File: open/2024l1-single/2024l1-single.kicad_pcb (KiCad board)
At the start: 2 copper layers, 176 x 169.5 mm, 100 parts, among them IC1 LM2587S-ADJ, J1 Conn_01x03, J2 Conn_01x03, J3 Conn_01x02, J4 Conn_01x02, J5 XT30, J6 Conn_01x04, Q1 STP75NF75, Q2 STP75NF75, U1 Seeed Studio XIAO SAMD21, U2 CD74HC4067SM

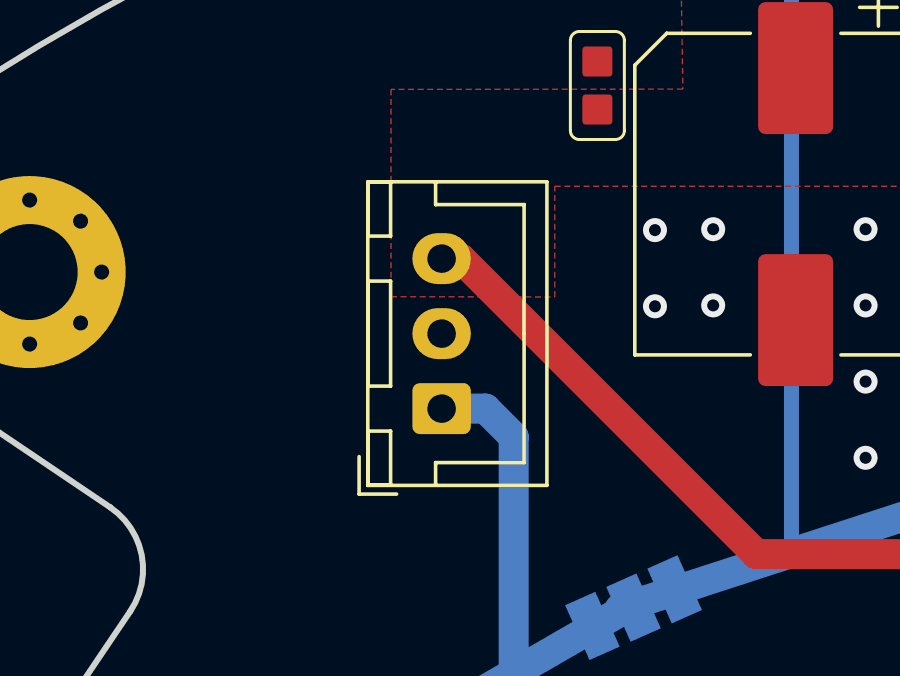
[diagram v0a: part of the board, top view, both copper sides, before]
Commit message: Connector movements
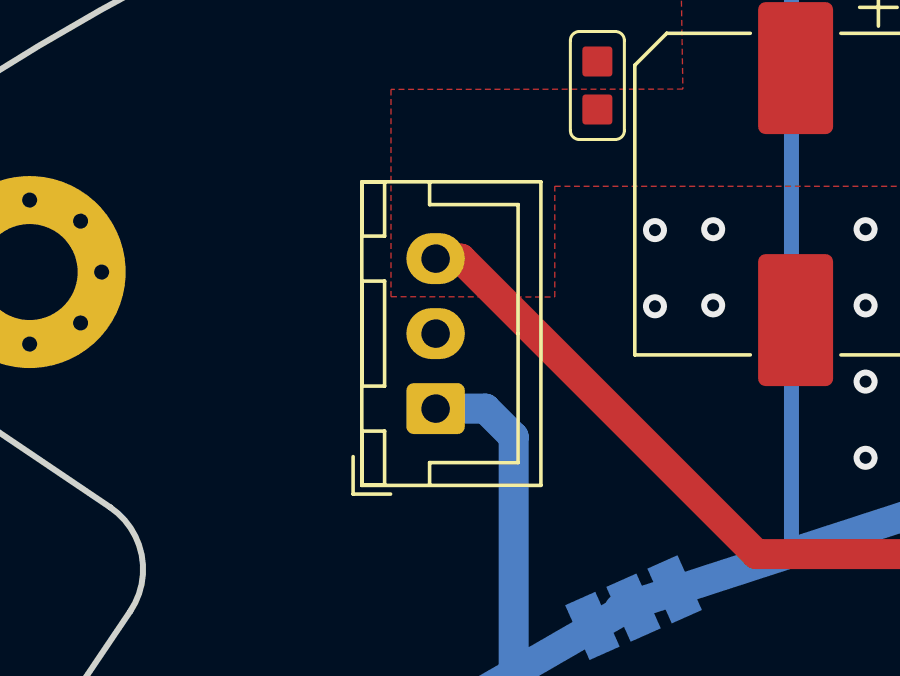
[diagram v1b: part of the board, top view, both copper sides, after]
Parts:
- moved J1 0.20 mm to (75.6, 48.8)
